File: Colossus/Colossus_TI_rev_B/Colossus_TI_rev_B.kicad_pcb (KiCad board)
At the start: 4 copper layers, 37.5 x 23 mm, 25 parts, among them J1 SWD, J2 MFC Connection Points, J3 Analog Debugging, J4 Power In, Q3 CSD18541F5, Q4 CSD18541F5, SW2 Reset, U1 XMSM0C1104SDYYR, U2 AD9833xRM, U3 MCP6L01Rx-xOT

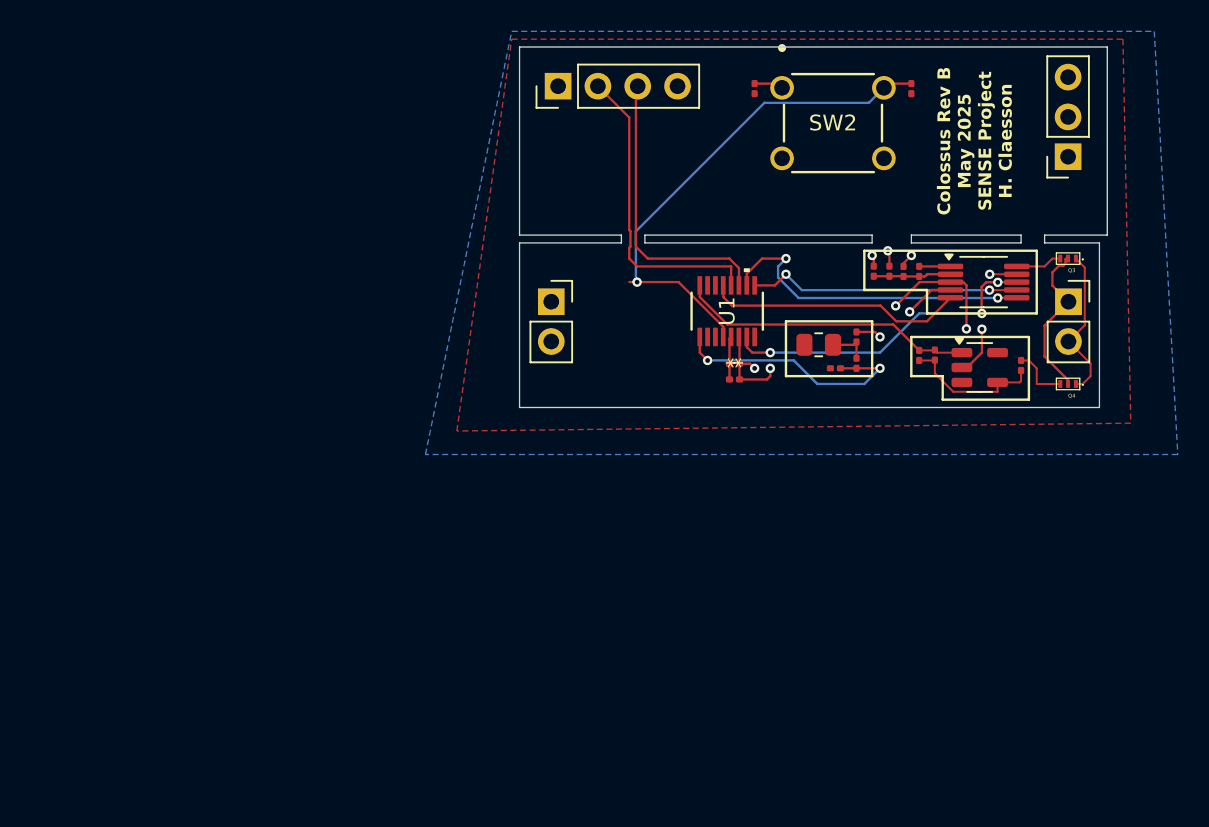
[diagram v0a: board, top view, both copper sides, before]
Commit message: working on miniaturization
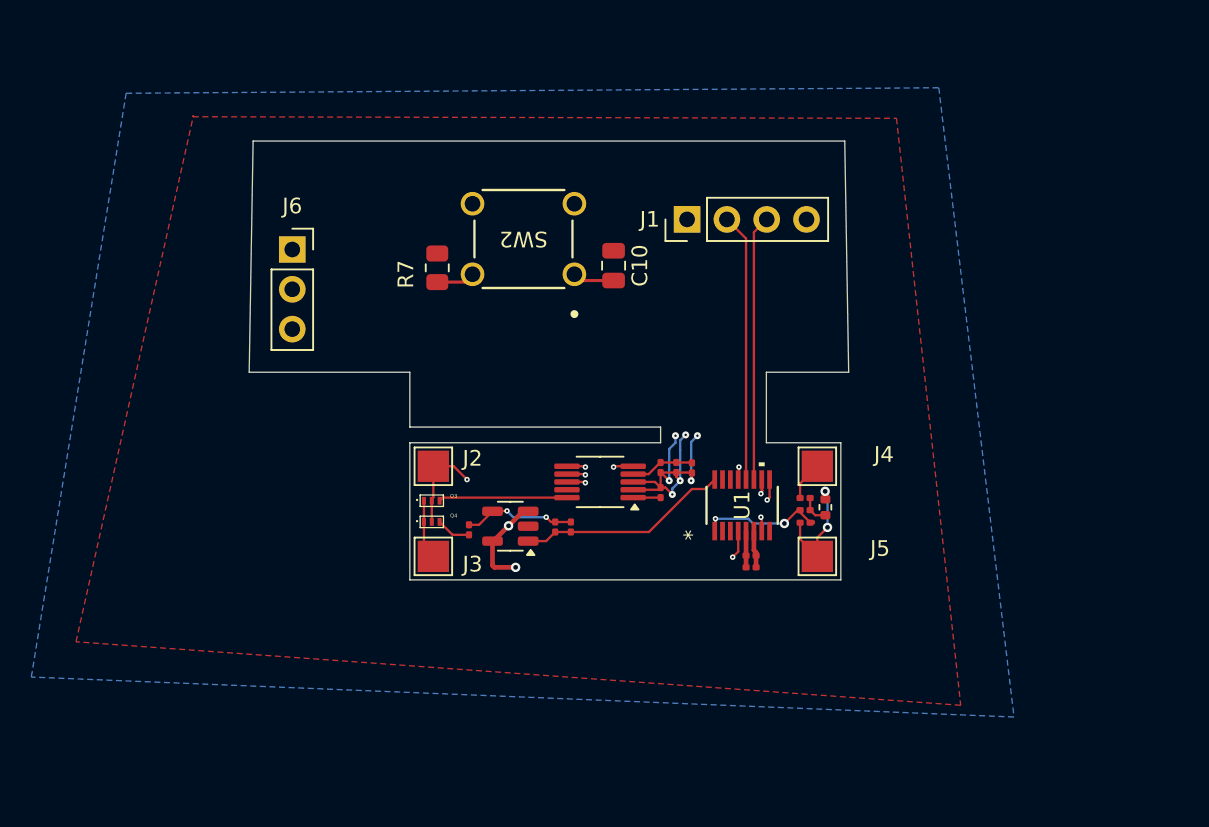
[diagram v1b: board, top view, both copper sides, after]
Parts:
- added J5: Power In (gnd), TestPoint:TestPoint_Pad_2.0x2.0mm, F.Cu at (109.0, 70.0)
- added J6: Analog Debugging, Connector_PinSocket_2.54mm:PinSocket_1x03_P2.54mm_Vertical, F.Cu at (75.5, 50.4)
- C10: footprint Capacitor_SMD:C_0201_0603Metric -> Capacitor_SMD:C_0805_2012Metric
- J2: value MFC Connection Points -> MFC GND; footprint Connector_PinSocket_2.54mm:PinSocket_1x02_P2.54mm_Vertical -> TestPoint:TestPoint_Pad_2.0x2.0mm
- J3: value Analog Debugging -> MFC V+; footprint Connector_PinSocket_2.54mm:PinSocket_1x03_P2.54mm_Vertical -> TestPoint:TestPoint_Pad_2.0x2.0mm
- J4: value Power In -> Power In (v+); footprint Connector_PinSocket_2.54mm:PinSocket_1x02_P2.54mm_Vertical -> TestPoint:TestPoint_Pad_2.0x2.0mm
- R7: footprint Resistor_SMD:R_0201_0603Metric -> Resistor_SMD:R_0805_2012Metric
- TH1: footprint Resistor_SMD:R_0805_2012Metric -> Resistor_SMD:R_0402_1005Metric
- moved J3 47.9 mm to (84.5, 70.0), turned to 0 degrees
- moved Q3 43.4 mm to (84.4, 66.5), turned to 0 degrees
- moved J2 41.9 mm to (84.5, 64.2)
- moved Q4 41.5 mm to (84.4, 67.8), turned to 0 degrees
- moved R3 36.8 mm to (86.8, 68.3), turned to 90 degrees
- moved R7 32.3 mm to (84.8, 51.6), turned to -90 degrees
- moved U3 31.6 mm to (89.4, 68.1), turned to 180 degrees
- moved U2 27.6 mm to (95.1, 65.2), turned to 180 degrees
- moved R4 26.6 mm to (92.3, 68.1), turned to -90 degrees
- moved C9 24.8 mm to (93.3, 68.1), turned to -90 degrees
- moved C4 21.7 mm to (99.0, 65.9), turned to 90 degrees
- moved J4 20.0 mm to (109.0, 64.2)
- moved C7 19.2 mm to (99.0, 64.3)
- moved C6 19.2 mm to (100.0, 64.3)
- moved SW2 17.8 mm to (93.5, 52.0), turned to 180 degrees
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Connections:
- J3 pad 1: A3 -> MFC IN
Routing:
- net Temp Read: track 16.3 -> 7.89 mm
- net FSYNC: track 20.9 -> 14.3 mm, vias 3 -> 2
- net SDATA: track 20.8 -> 14.6 mm
- net MFC IN: track 9.89 -> 3.80 mm
- net Strain Read: track 19.0 -> 13.5 mm
- net FMout: track 2.98 -> 8.21 mm
- net 24MHzClockOut: track 16.5 -> 11.9 mm, vias 0 -> 2
- net NRST: track 32.6 -> 36.7 mm
- net Vdd: track 20.6 -> 24.6 mm, vias 4 -> 7
- net SWCLK: track 19.8 -> 17.1 mm
- net Vss: track 24.3 -> 26.5 mm, vias 7 -> 5
- net SCLK: track 17.4 -> 15.2 mm
- net Net-(U3--): track 9.15 -> 7.16 mm, vias 0 -> 2
- net SWDIO: track 18.5 -> 16.9 mm
- net Charge Amp In: track 3.71 -> 2.22 mm
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- added copper zone on In2.Cu, net Vss
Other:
- board size 37.5 x 23 mm -> 38.2 x 28 mm
- board text removed: "Colossus Rev B May 2025 SENSE Project H. Claesson"

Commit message: pushing to take the trian to family day
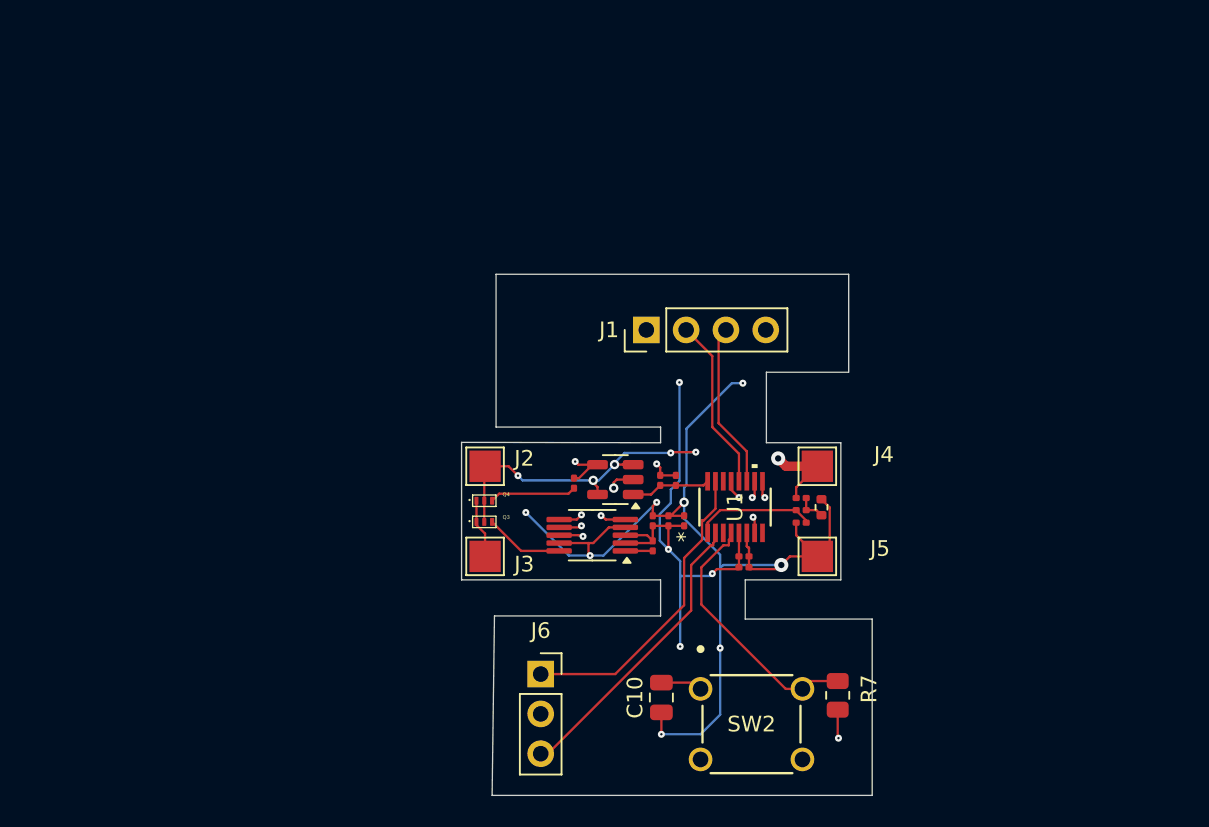
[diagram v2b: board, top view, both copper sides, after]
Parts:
- moved R7 37.4 mm to (110.3, 78.9), turned to 90 degrees
- moved J6 31.4 mm to (91.3, 77.5)
- moved C10 27.7 mm to (99.0, 79.0), turned to 90 degrees
- moved SW2 27.7 mm to (101.5, 78.5), turned to 0 degrees
- moved J1 7.51 mm to (98.1, 55.5)
- moved U3 7.33 mm to (96.1, 65.1)
- moved R3 7.33 mm to (93.5, 65.3)
- moved C9 7.33 mm to (100.0, 65.2)
- moved R4 7.33 mm to (99.0, 65.2)
- moved Q3 3.61 mm to (87.8, 67.8)
- moved Q4 3.61 mm to (87.8, 66.5)
- moved C6 3.44 mm to (99.5, 67.7)
- moved C7 3.44 mm to (98.5, 67.7)
- moved U2 3.44 mm to (94.6, 68.7)
- moved C4 3.44 mm to (98.5, 69.3)
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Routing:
- net Vss: track 26.5 -> 93.5 mm, vias 5 -> 13
- net Vdd: track 24.6 -> 45.5 mm
- net NRST: track 36.7 -> 16.7 mm, vias 1 -> 0
- net A3: track 0.00 -> 19.8 mm
- net A5: track 0.00 -> 19.1 mm
- net Strain Read: track 13.5 -> 5.10 mm
- net SWDIO: track 16.9 -> 10.6 mm
- net SWCLK: track 17.1 -> 11.1 mm
- net Net-(U3--): track 7.16 -> 10.9 mm
- net Charge Amp In: track 2.22 -> 5.56 mm
- net FMout: track 8.21 -> 5.04 mm
- net 24MHzClockOut: track 11.9 -> 12.6 mm
- net Temp Read: track 7.89 -> 7.80 mm, vias 2 -> 0
- added copper zone on In2.Cu, net Vdd
- removed copper zone on F.Cu, net Vdd
- removed copper zone on B.Cu, net Vss
- removed copper zone on In2.Cu, net Vss
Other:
- board size 38.2 x 28 mm -> 26.2 x 33.2 mm

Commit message: final and manufactured draft of revB board
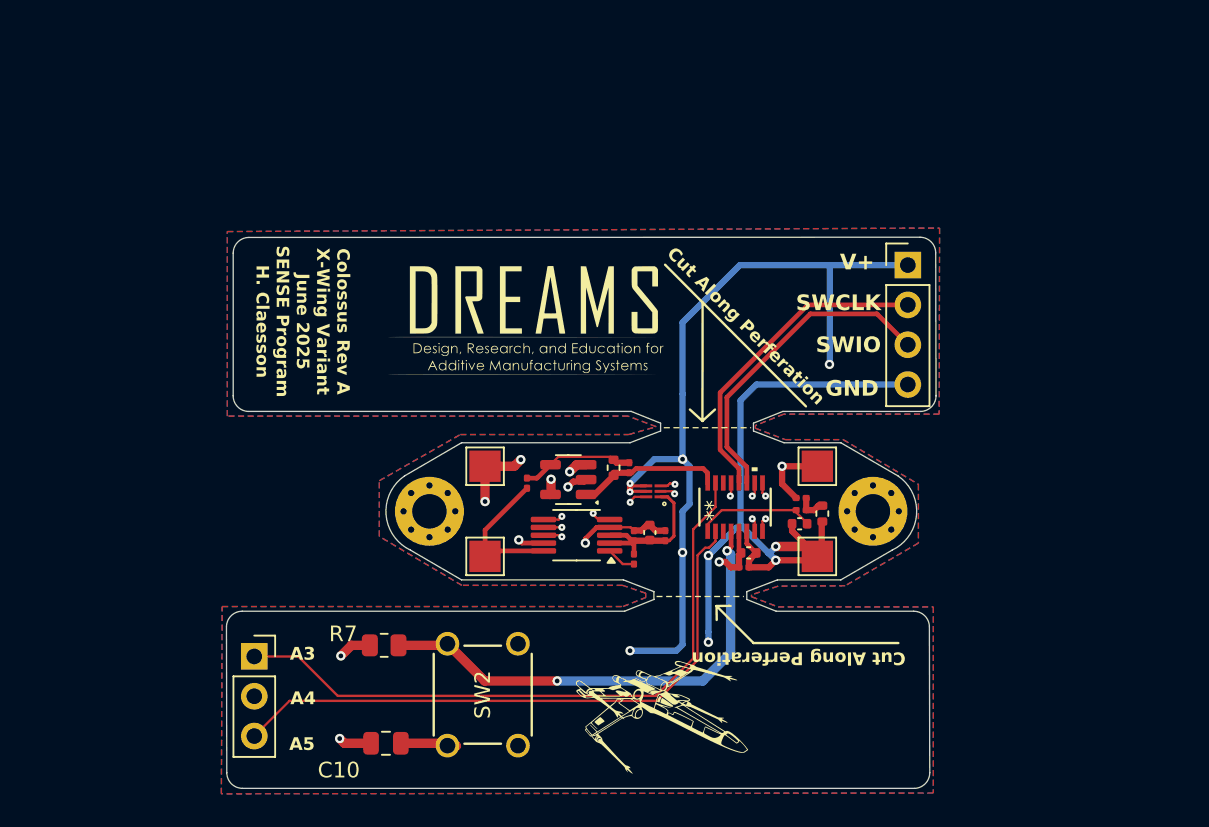
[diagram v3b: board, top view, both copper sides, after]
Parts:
- removed Q3, Q4: CSD18541F5, CSD18541F5 - n channel mosfet:DFN149X73X35-3N
- added G***: LOGO, DreamsLabLogo:dreamslogo, F.Cu at (91.2, 54.9)
- added G***: LOGO, xwing:xwing3, F.Cu at (99.1, 80.3)
- added H1: MountingHole, MountingHole:MountingHole_2.2mm_M2_Pad_Via, F.Cu at (84.2, 67.1)
- added H2: MountingHole, MountingHole:MountingHole_2.2mm_M2_Pad_Via, F.Cu at (112.5, 67.1)
- added U4: SN74LVC1G3157DSFR, Analog Switch - SN74LVC1G3157DSFR:SON35P100X100X40-6N, F.Cu at (98.5, 65.8)
- C1, C6, C8: footprint Capacitor_SMD:C_0201_0603Metric -> Capacitor_SMD:C_0402_1005Metric
- R4: footprint Resistor_SMD:R_0201_0603Metric -> Resistor_SMD:R_0402_1005Metric
- SW2: footprint button:SW_B3F-1000_OMR -> footprints:SW_B3F-1000_OMR
- U1: footprint footprints:SOT-23-THIN16_DYY_TEX-M -> MSMP0:SOT-23-THIN16_DYY_TEX
- moved R7 29.1 mm to (81.4, 75.7), turned to 0 degrees
- moved J6 18.3 mm to (73.1, 76.4)
- moved C10 17.8 mm to (81.5, 81.9), turned to 0 degrees
- moved J1 17.2 mm to (114.8, 51.4), turned to 0 degrees
- moved SW2 16.6 mm to (85.4, 82.1), turned to 90 degrees
- moved C9 3.08 mm to (97.0, 64.3)
- moved R4 3.08 mm to (96.0, 64.3)
- moved R3 3.00 mm to (90.5, 65.3)
- moved U3 3.00 mm to (93.1, 65.1)
- moved C5 1.53 mm to (99.3, 68.7)
- moved C7 1.53 mm to (97.3, 68.7)
- moved C4 1.46 mm to (97.3, 70.2)
- moved C6 1.41 mm to (98.3, 68.5)
- moved U2 1.00 mm to (93.6, 68.7)
- moved TH1 0.41 mm to (109.3, 67.3), turned to 90 degrees
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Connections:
- C4 pad 2: Vdd -> FM Power
- C5 pad 2: Vdd -> FM Power
- C6 pad 2: Vdd -> FM Power
- C7 pad 1: Vdd -> FM Power
- J3 pad 1: MFC IN -> Charge Amp In
- U1 pad 8: PA2 -> Mode Select
- U2 pad 10: FMout -> Charge Amp In
- U2 pad 2: Vdd -> FM Power
- U2 pad 3: Vdd -> FM Power
- U3 pad 2: Vdd -> Strain Power
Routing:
- net Vss: track 93.5 -> 64.6 mm, vias 13 -> 12
- net Vdd: track 45.5 -> 73.3 mm, vias 7 -> 9
- net A3: track 19.8 -> 41.8 mm
- net A5: track 19.1 -> 39.1 mm
- net NRST: track 16.7 -> 30.9 mm, vias 0 -> 2
- net Mode Select: track 0.00 -> 10.9 mm, vias 0 -> 2
- net SWDIO: track 10.6 -> 20.6 mm
- net FM Power: track 0.00 -> 9.95 mm
- net Strain Power: track 0.00 -> 9.61 mm, vias 0 -> 2
- net SWCLK: track 11.1 -> 20.6 mm
- net FMout: track 5.04 -> 0.00 mm
- net Strain Read: track 5.10 -> 9.12 mm
- net MFC IN: track 3.78 -> 0.00 mm
- net Charge Amp In: track 5.56 -> 9.33 mm
- net Net-(U3--): track 10.9 -> 7.57 mm, vias 2 -> 0
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- added copper zone on F.Cu, net Vdd
- added copper zone on B.Cu, net Vss
- added copper zone on In1.Cu, net Vss
- added copper zone on In2.Cu, net Vss
- removed copper zone on In2.Cu, net Vdd
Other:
- board size 26.2 x 33.2 mm -> 45.3 x 35.2 mm
- board text added: "A3"
- board text added: "A4"
- board text added: "A5"
- board text added: "Colossus Rev A X-Wing Variant June 2025 SENSE Program H. Claesson"
- board text added: "Cut Along Perferation"
- board text added: "Debugging"
- board text added: "GND"
- board text added: "Programming"
- board text added: "SWCLK"
- board text added: "SWIO"
- board text added: "V+"
